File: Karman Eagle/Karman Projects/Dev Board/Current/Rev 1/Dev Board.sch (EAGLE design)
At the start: 59 parts, among them J1 I2C1, J10 P8-P13, J11 47219-2001, J2 P0-P3, J3 A0-A3, J4 Debug, J5 P4-P7, J6 VCC, J7 GND, J8 SPI1, J9 UART5, U1 BNO055, U2 ADXL377, U3 BNO055

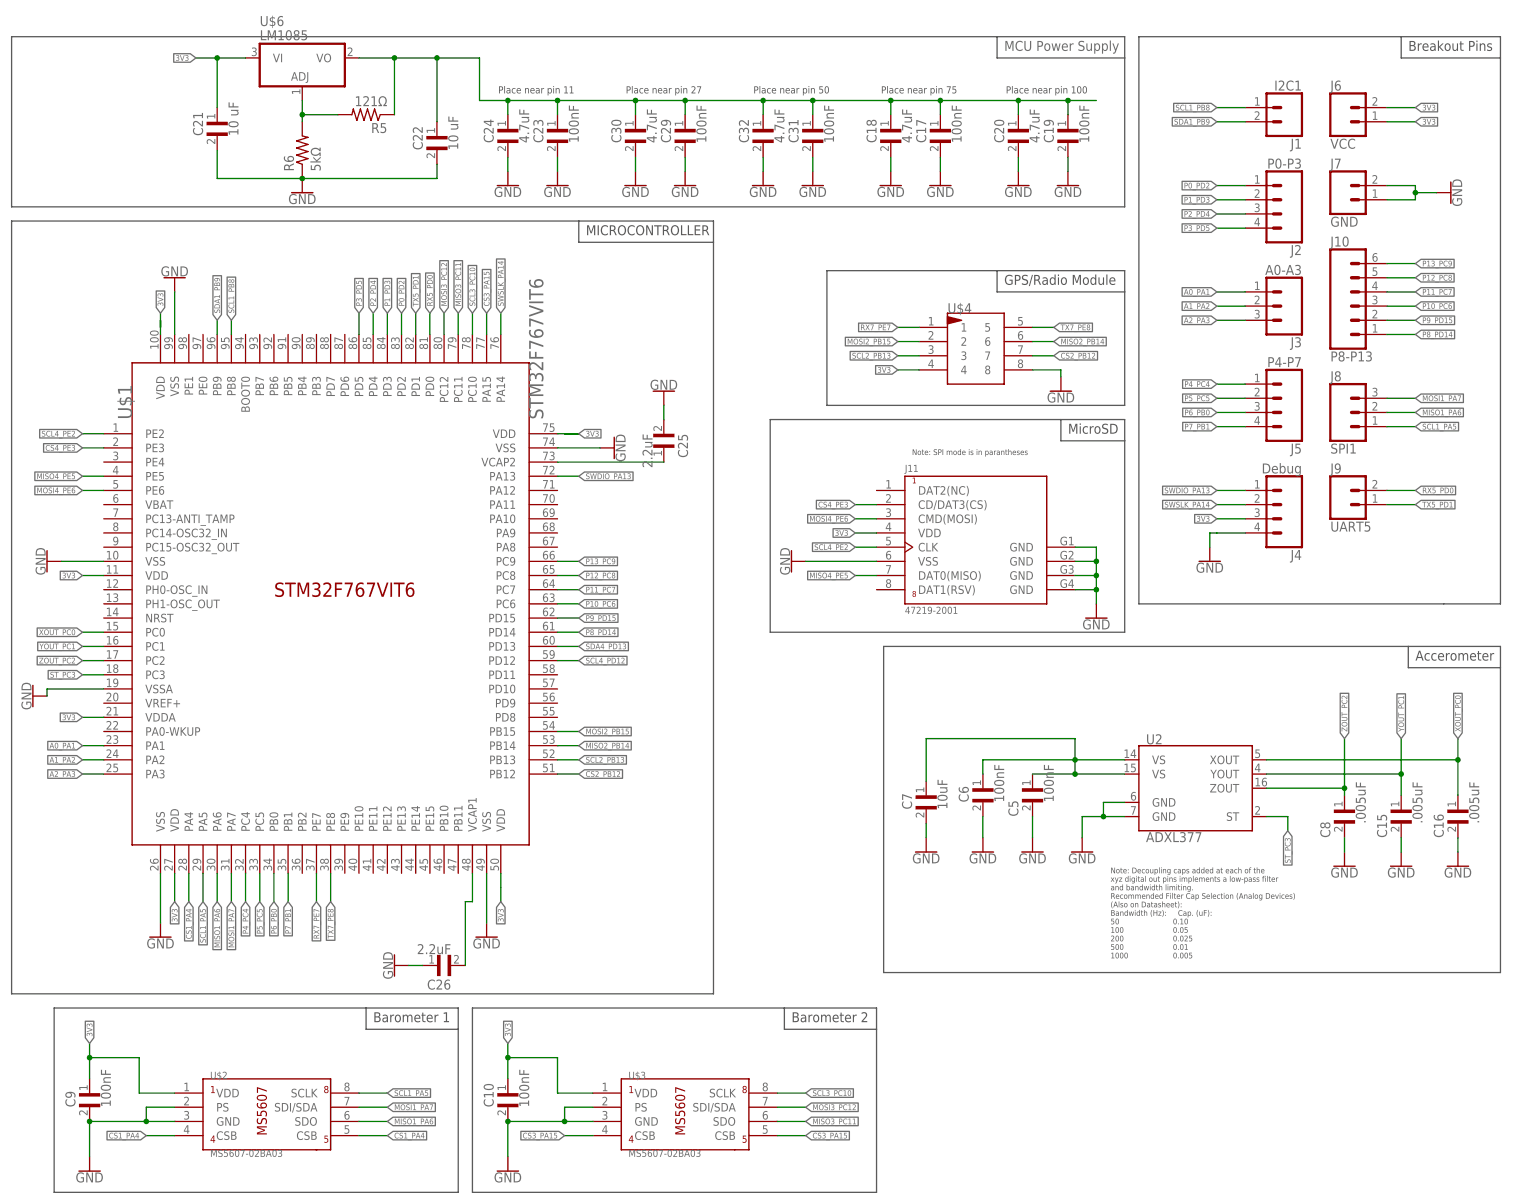
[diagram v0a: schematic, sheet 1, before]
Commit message: 5/25/19 11:45 PCB Issued for Review
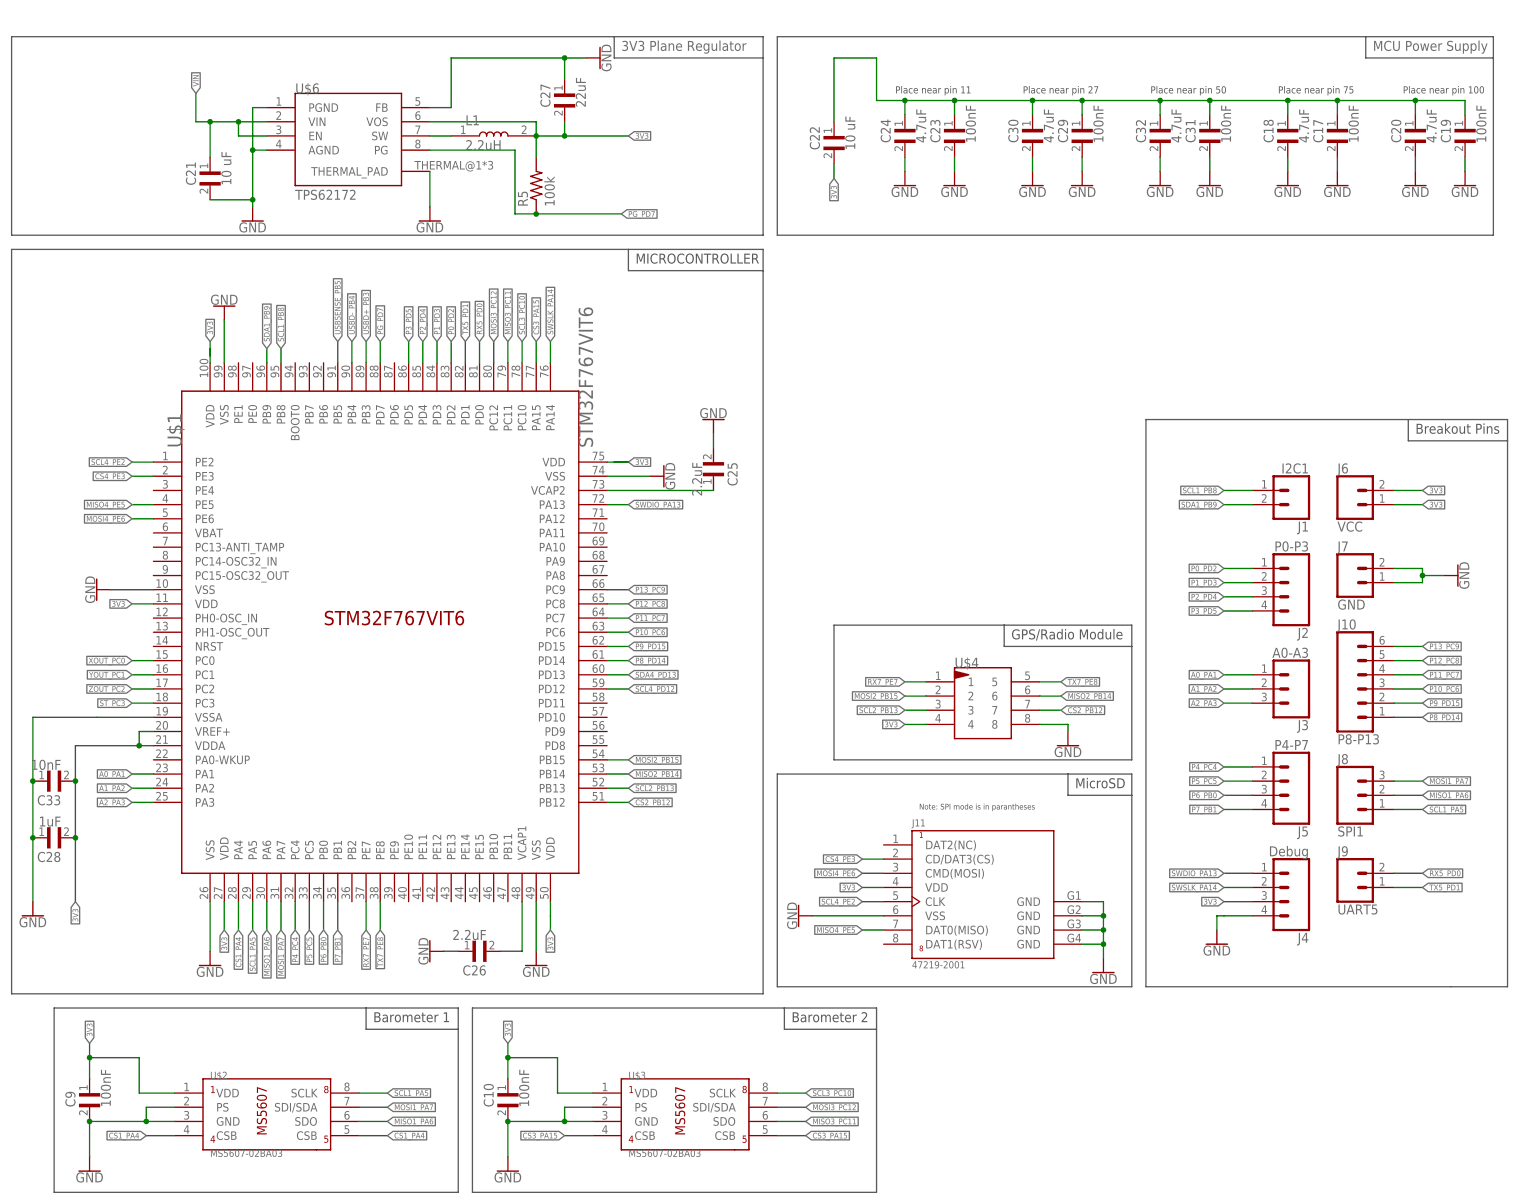
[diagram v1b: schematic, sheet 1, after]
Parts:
- added C27: 22uF, CGA3E2X7R1H104K080AD:CGA3E2X7R1H104K080AD
- added C28: 1uF, CGA3E2X7R1H104K080AD:CGA3E2X7R1H104K080AD
- added C33: 10nF, CGA3E2X7R1H104K080AD:CGA3E2X7R1H104K080AD
- added C34: 4.7nF, CGA3E2X7R1H104K080AD:CGA3E2X7R1H104K080AD
- added J12: 105164-0001, 105164-0001:105164-0001
- added L1: 2.2uH, 0603_Inductor:MLF1608E100J
- added R7: 59k, 0603_Resistor:CRGH0603F221K
- added R8: 42.2k, 0603_Resistor:CRGH0603F221K
- added U$10, U$11, U$7, U$8, U$9: PESD3V3S1UL, PESD3V3S1UL:PESD3V3S1UL
- R5: value 121Ω -> 100k; device CRGH0603F221K:CRGH0603F221K -> 0603_Resistor:CRGH0603F221K
- R6: value 5kΩ -> 1M; device CRGH0603F221K:CRGH0603F221K -> 0603_Resistor:CRGH0603F221K
- U$6: value LM1085 -> TPS62172; device LM1085:LM1085 -> TPS62172:TPS62172
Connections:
- removed net N$9: C21.2, C22.2, R6.1
- new net N$13: J12.ID
- new net N$14: C34.2, J12.SHIELD, R6.1, U$10.CA, U$11.CA, U$9.CA
- new net PG_PD7: R5.1, U$1.PD7, U$6.PG
- new net USBD+_PB3: J12.D+, U$1.PB3, U$11.AN, U$8.CA
- new net USBD-_PB4: J12.D-, U$1.PB4, U$10.AN, U$7.CA
- new net USBSENSE_PB5: R7.2, R8.1, U$1.PB5
- new net VIN: C21.1, J12.5V_IN, R8.2, U$6.EN, U$6.VIN, U$7.AN, U$8.AN, U$9.AN
- net 3V3: now also C22.2, C27.2, C28.2, C33.2, L1.2, R5.2, U$1.VREF+, U$6.VOS; no longer C21.1, U$6.VI
- net GND: now also C21.2, C27.1, C28.1, C33.1, C34.1, J12.GND, R6.2, R7.1, U$6.AGND, U$6.FB, U$6.PGND, U$6.THERMAL_PAD
- net N$10: no longer R5.1, U$6.VO
- net N$8: now also L1.1, U$6.SW; no longer R5.2, R6.2, U$6.ADJ
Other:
- note added: "3V3 Plane Regulator"
- note added: "Micro USB"
- moved on the sheet: C17, C18, C19, C20, C21, C22, C23, C24, C25, C26, C29, C30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

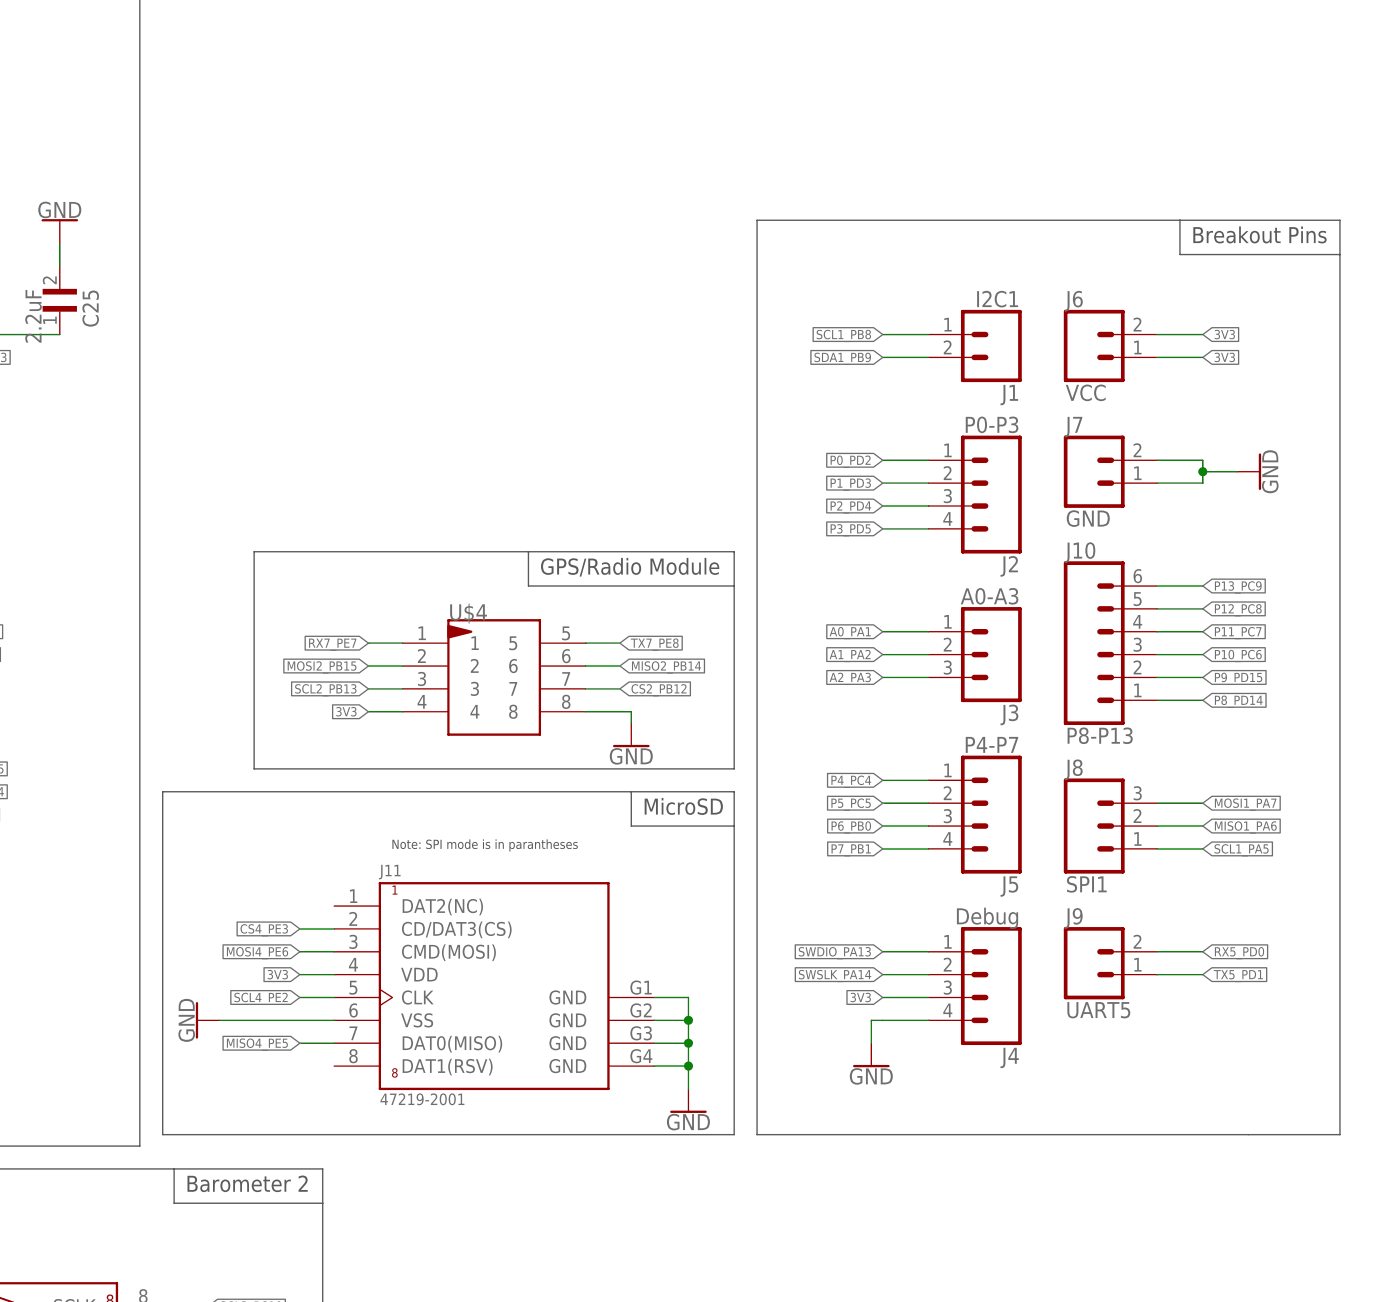
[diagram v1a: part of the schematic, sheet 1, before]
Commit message: 5/25/19 12:47 PCB ISSUED FOR REVIEW
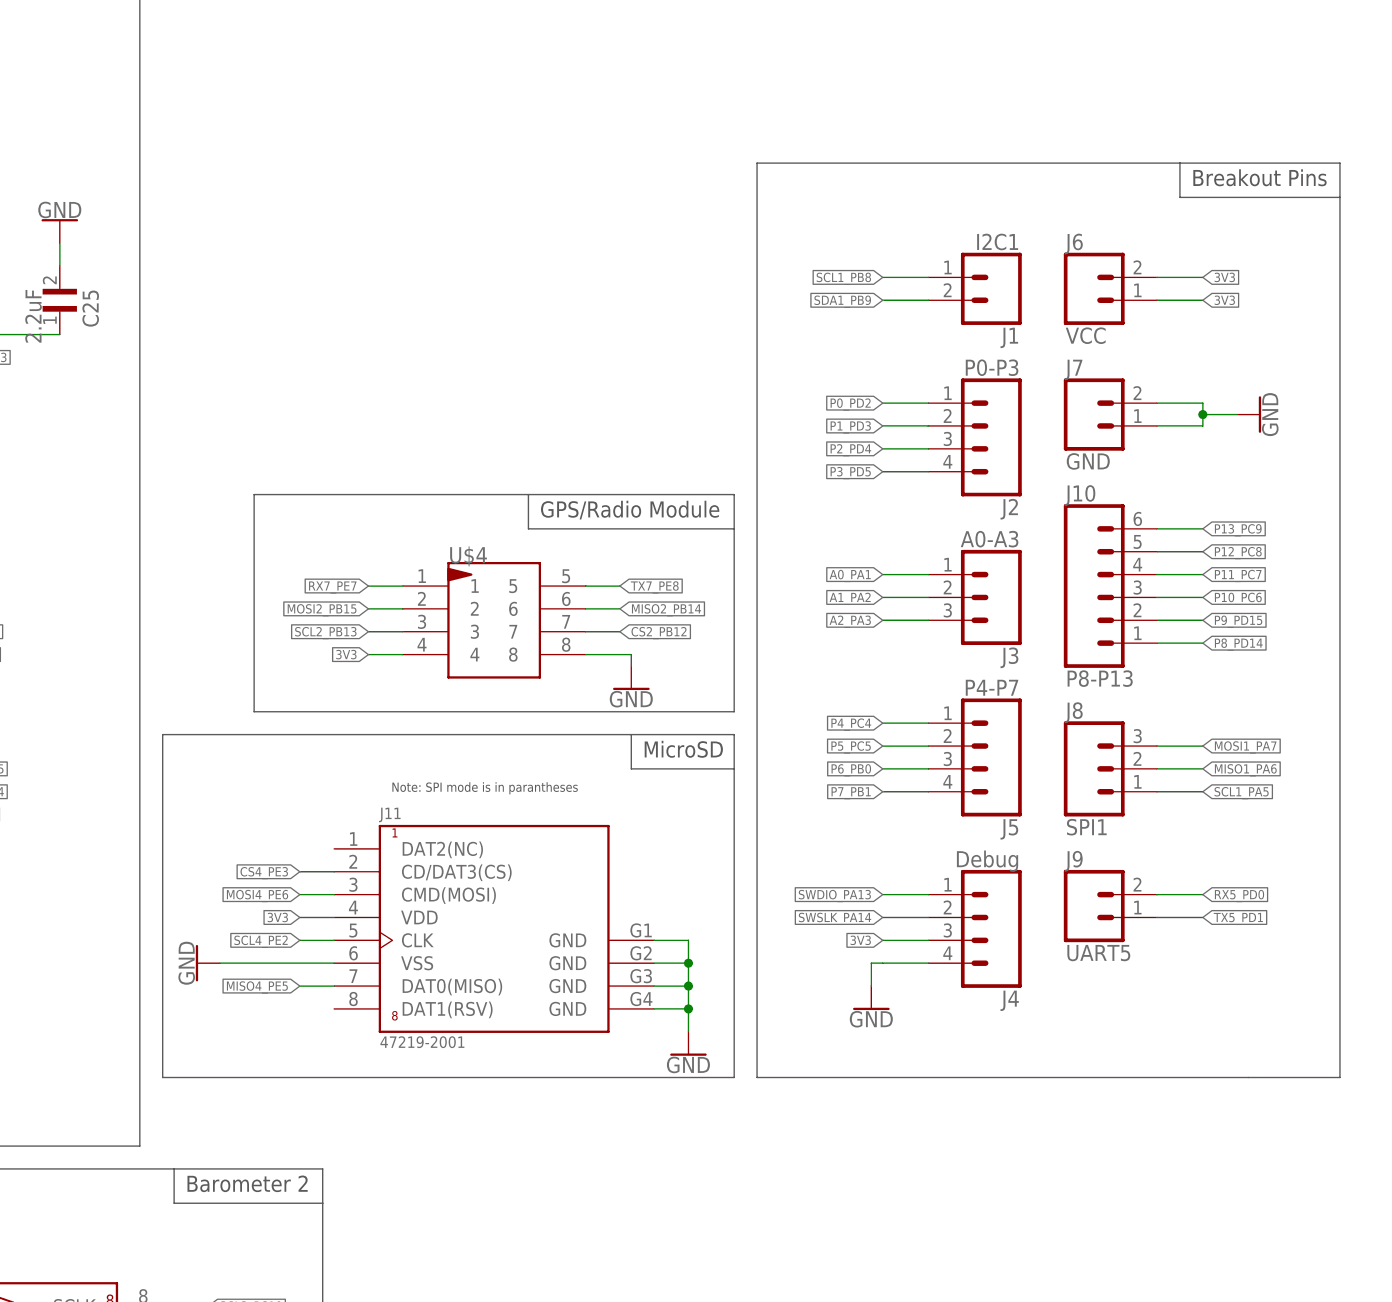
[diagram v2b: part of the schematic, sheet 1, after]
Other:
- moved on the sheet: J1, J10, J11, J2, J3, J4, J5, J6, J7, J8, J9, U$4
